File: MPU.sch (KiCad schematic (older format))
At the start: 19 parts, among them J2 Conn_02x10_Counter_Clockwise, J3 Micro_SD_Card, J4 USB_A, J5 USB_A, SW1 SW_DIP_x03, U1 STM32MP151AAB3, Y1 Crystal_GND24, Y2 Crystal_GND24

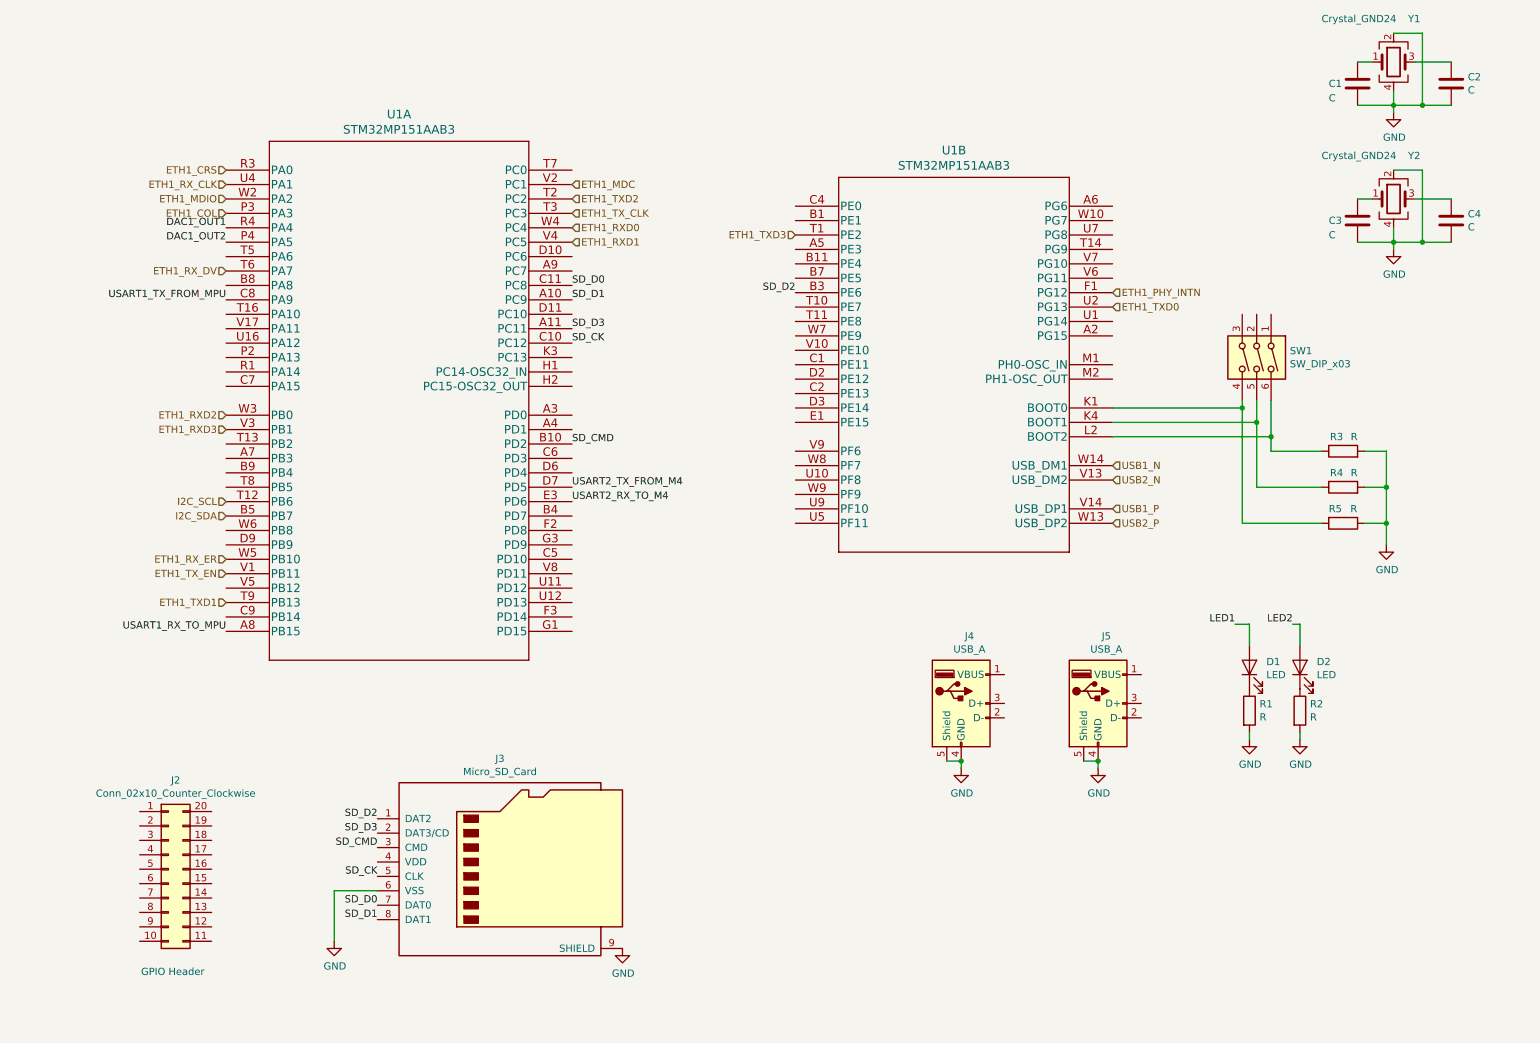
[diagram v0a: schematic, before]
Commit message: Finish labelling RAM
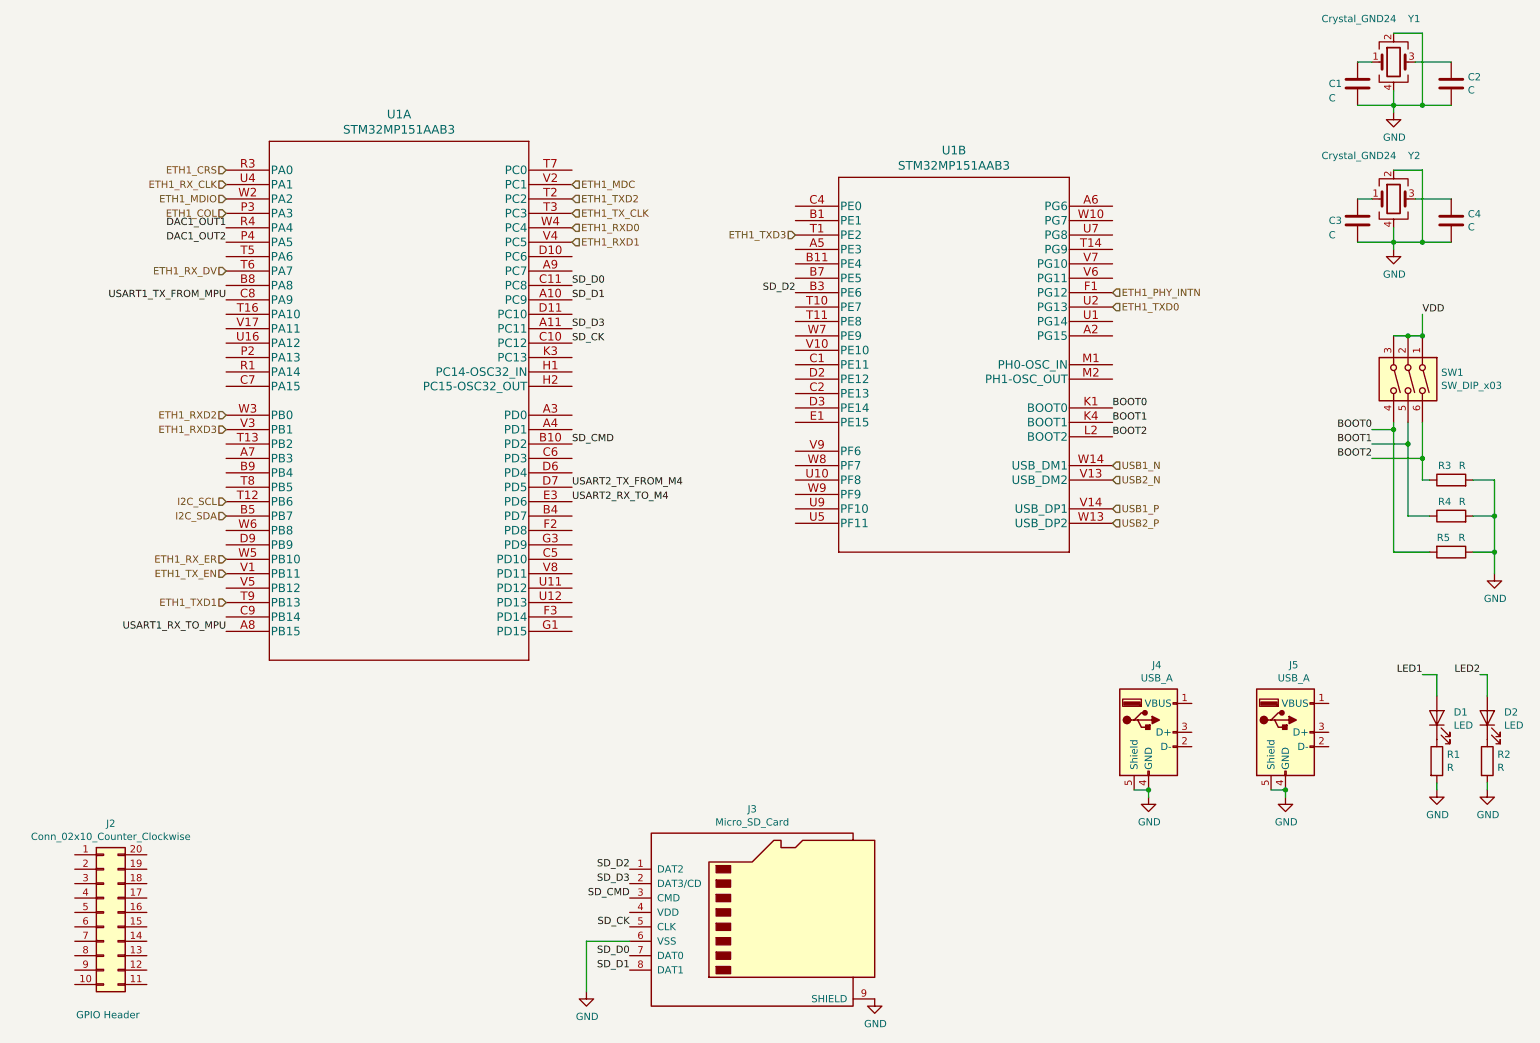
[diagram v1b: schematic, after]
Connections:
- net BOOT0: now reaches R5.2, SW1.4, U1.K1 (BOOT0)
- net BOOT1: now reaches R4.1, SW1.5, U1.K4 (BOOT1)
- net BOOT2: now reaches R3.1, SW1.6, U1.L2 (BOOT2)
- net VDD: now reaches SW1.1
- net VDD: now also SW1.2, SW1.3
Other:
- moved on the sheet: D1, D2, J2, J3, J4, J5, R1, R2, R3, R4, R5, SW1
